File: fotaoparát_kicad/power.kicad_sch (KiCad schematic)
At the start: 63 parts

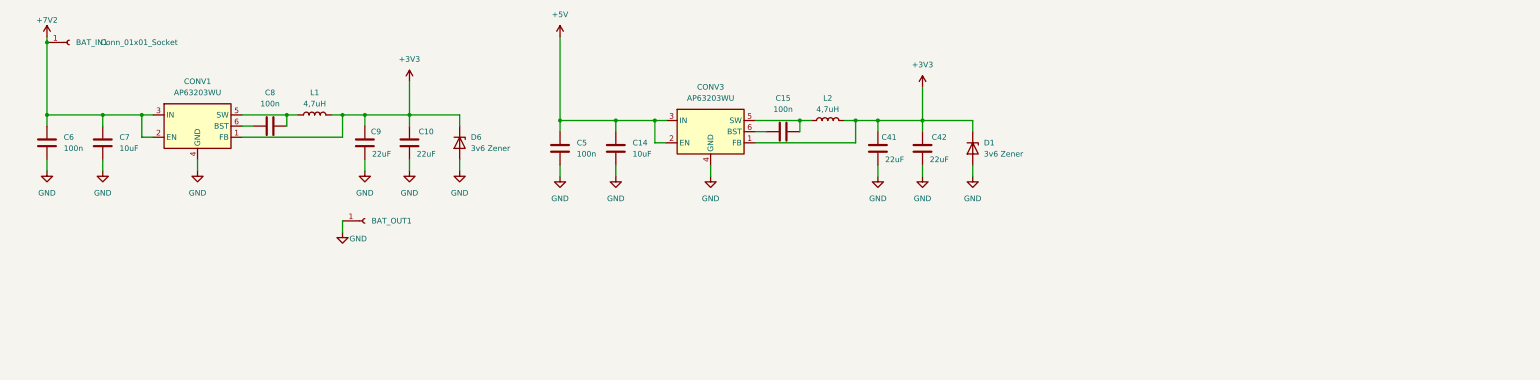
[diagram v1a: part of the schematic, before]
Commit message: XDD NEVIM ZABIJU SE
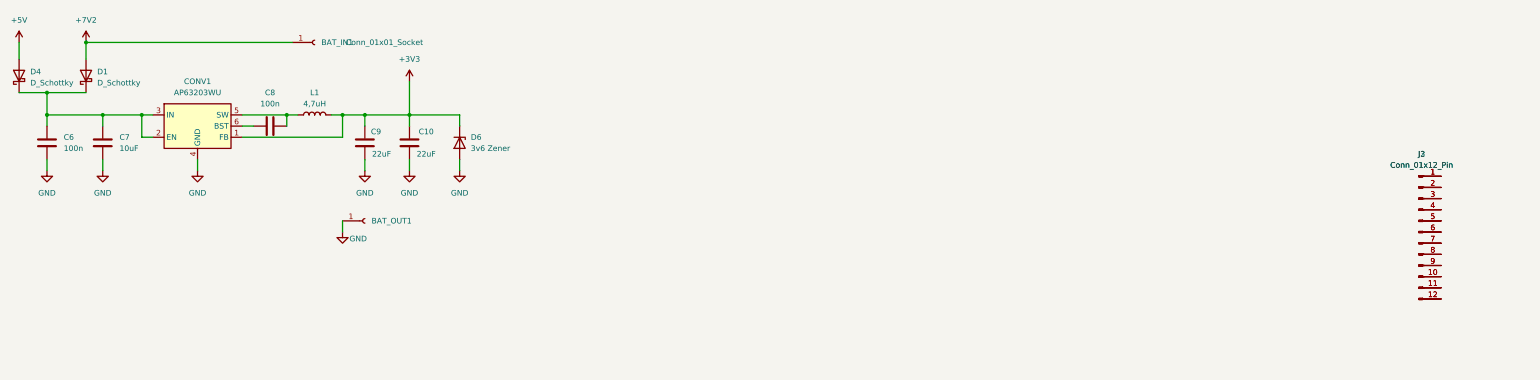
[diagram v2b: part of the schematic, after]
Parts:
- removed C14: 10uF, Capacitor_SMD:C_0603_1608Metric, symbol Device:C
- removed C15, C5: 100n, Capacitor_SMD:C_0603_1608Metric, symbol Device:C
- removed C41, C42: 22uF, Capacitor_SMD:C_0603_1608Metric, symbol Device:C
- removed CONV3: AP63203WU, Package_TO_SOT_SMD:TSOT-23-6, symbol Regulator_Switching:AP63203WU
- removed D1: 3v6 Zener, Diode_SMD:D_SOD-123, symbol Device:D_Zener
- removed L2: 4,7uH, Inductor_SMD:L_0603_1608Metric, symbol Device:L
- added D1, D4: D_Schottky, Diode_SMD:D_0805_2012Metric, symbol Device:D_Schottky
- added J2: Conn_01x12_Pin, Connector_FFC-FPC:Hirose_FH12-11S-0.5SH_1x11-1MP_P0.50mm_Horizontal, symbol Connector:Conn_01x12_Pin
- added J3: Conn_01x12_Pin, symbol Connector:Conn_01x12_Pin
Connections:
- net +5V: now also D4.2 (A)
- net +7V2: now also D1.2 (A); no longer C6.2, C7.2, CONV1.2 (EN), CONV1.3 (IN)
- new net: C6.2, C7.2, CONV1.2 (EN), CONV1.3 (IN), D1.1 (K), D4.1 (K)
- new net: J2.1 (Pin_1), J3.1 (Pin_1)
- new net: J2.10 (Pin_10), J3.10 (Pin_10)
- new net: J2.11 (Pin_11), J3.11 (Pin_11)
- new net: J2.12 (Pin_12), J3.12 (Pin_12)
- new net: J2.2 (Pin_2), J3.2 (Pin_2)
- new net: J2.3 (Pin_3), J3.3 (Pin_3)
- new net: J2.4 (Pin_4), J3.4 (Pin_4)
- new net: J2.5 (Pin_5), J3.5 (Pin_5)
- new net: J2.6 (Pin_6), J3.6 (Pin_6)
- new net: J2.7 (Pin_7), J3.7 (Pin_7)
- new net: J2.8 (Pin_8), J3.8 (Pin_8)
- new net: J2.9 (Pin_9), J3.9 (Pin_9)
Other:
- moved on the sheet: BAT_IN1
